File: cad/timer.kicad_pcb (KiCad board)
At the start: 2 copper layers, 47 x 47 mm, 29 parts, among them Q1 BS170, Q2 BS170, U1 ATMEGA328P-PU, U2 LM393, Y1 32.768kHz

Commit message: Further changes from latest KiCad version
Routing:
- net Net-(C8-Pad1): track 8.41 -> 7.56 mm
- net Net-(C9-Pad1): track 8.41 -> 7.57 mm
- net GND: track 34.4 -> 33.9 mm
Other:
- net class Default removed

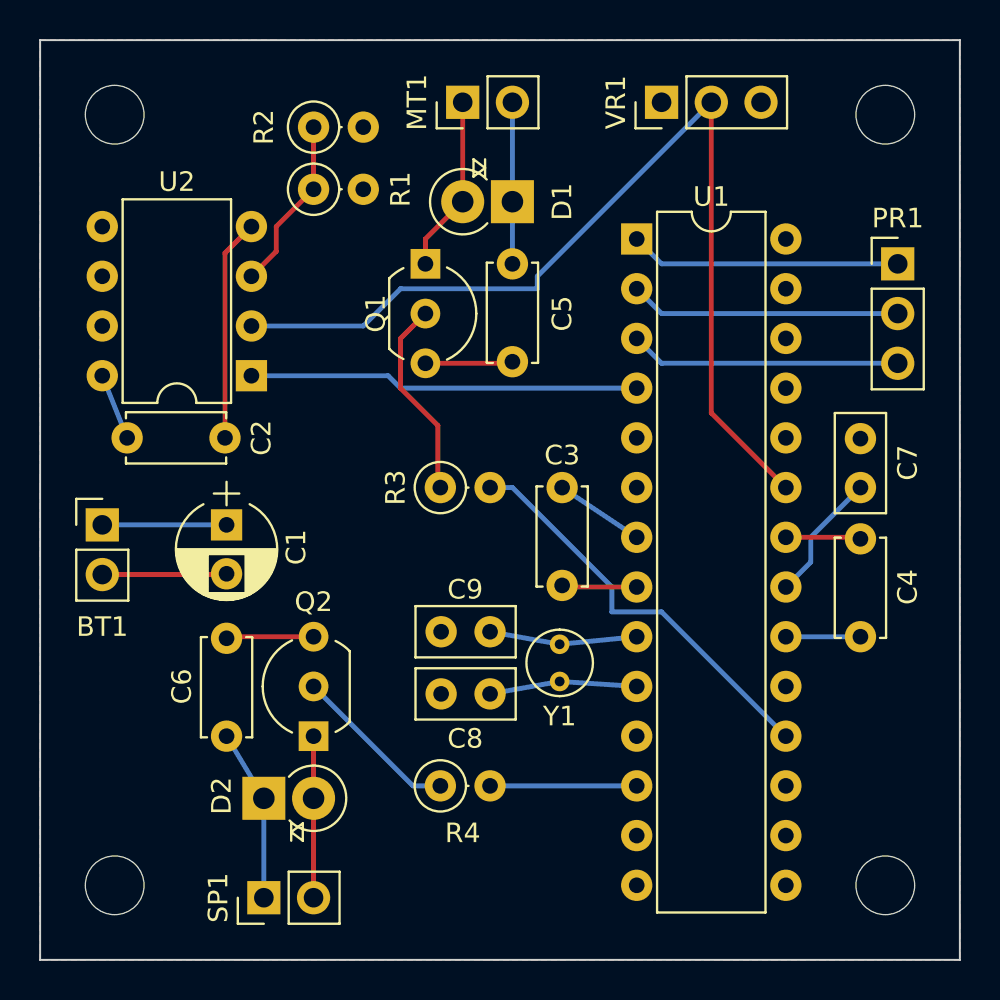
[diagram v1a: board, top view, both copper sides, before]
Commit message: Update CAD for redesign
Also cleanup old files in cad directory
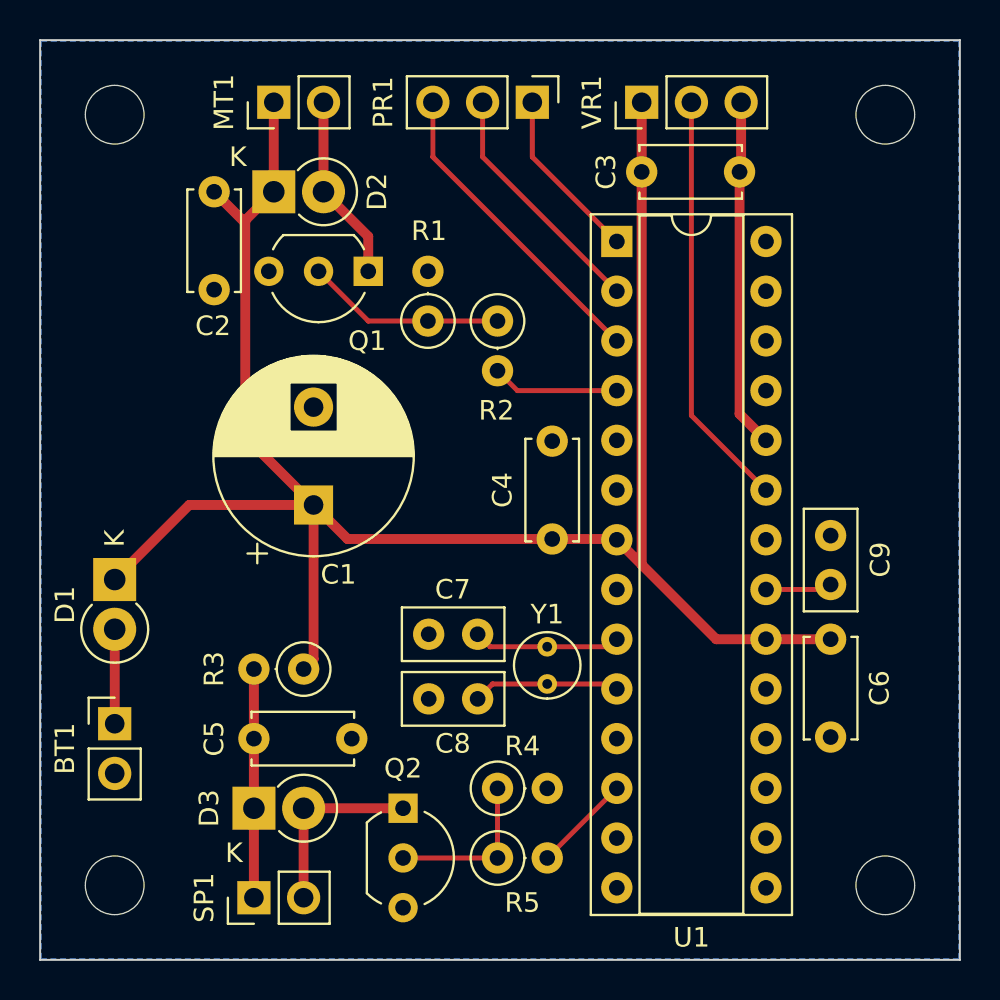
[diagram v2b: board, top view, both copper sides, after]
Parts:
- removed the C2 at (126.4, 89.5)
- removed the R2 at (135.9, 73.7)
- removed U2: LM393, Housings_DIP:DIP-8_W7.62mm
- added C3: 100nF, Capacitor_THT:C_Disc_D5.0mm_W2.5mm_P5.00mm, F.Cu at (152.7, 75.9)
- added D1: 1N5819, Diode_THT:D_DO-41_SOD81_P2.54mm_Vertical_KathodeUp, F.Cu at (125.7, 96.8)
- added R3: 4.7Ω, Resistor_THT:R_Axial_DIN0207_L6.3mm_D2.5mm_P2.54mm_Vertical, F.Cu at (135.4, 101.3)
- added R4: 100kΩ, Resistor_THT:R_Axial_DIN0207_L6.3mm_D2.5mm_P2.54mm_Vertical, F.Cu at (145.3, 107.4)
- BT1, MT1, SP1: footprint Pin_Headers:Pin_Header_Straight_1x02_Pitch2.54mm -> Connector_PinHeader_2.54mm:PinHeader_1x02_P2.54mm_Vertical
- C1: value 10uF -> 470µF; footprint Capacitors_THT:CP_Radial_D5.0mm_P2.50mm -> Capacitor_THT:CP_Radial_D10.0mm_P5.00mm
- C2: renamed from C5; footprint Capacitors_THT:C_Disc_D5.0mm_W2.5mm_P5.00mm -> Capacitor_THT:C_Disc_D5.0mm_W2.5mm_P5.00mm
- C4: renamed from C3; footprint Capacitors_THT:C_Disc_D5.0mm_W2.5mm_P5.00mm -> Capacitor_THT:C_Disc_D5.0mm_W2.5mm_P5.00mm
- C5: renamed from C6; footprint Capacitors_THT:C_Disc_D5.0mm_W2.5mm_P5.00mm -> Capacitor_THT:C_Disc_D5.0mm_W2.5mm_P5.00mm
- C6: renamed from C4; footprint Capacitors_THT:C_Disc_D5.0mm_W2.5mm_P5.00mm -> Capacitor_THT:C_Disc_D5.0mm_W2.5mm_P5.00mm
- C7: renamed from C9; footprint Capacitors_THT:C_Disc_D5.0mm_W2.5mm_P2.50mm -> Capacitor_THT:C_Disc_D5.0mm_W2.5mm_P2.50mm
- C8: footprint Capacitors_THT:C_Disc_D5.0mm_W2.5mm_P2.50mm -> Capacitor_THT:C_Disc_D5.0mm_W2.5mm_P2.50mm
- C9: renamed from C7; footprint Capacitors_THT:C_Disc_D5.0mm_W2.5mm_P2.50mm -> Capacitor_THT:C_Disc_D5.0mm_W2.5mm_P2.50mm
- D2: renamed from D1; footprint Diodes_THT:D_DO-41_SOD81_P2.54mm_Vertical_KathodeUp -> Diode_THT:D_DO-41_SOD81_P2.54mm_Vertical_KathodeUp
- D3: renamed from D2; footprint Diodes_THT:D_DO-41_SOD81_P2.54mm_Vertical_KathodeUp -> Diode_THT:D_DO-41_SOD81_P2.54mm_Vertical_KathodeUp
- PR1, VR1: footprint Pin_Headers:Pin_Header_Straight_1x03_Pitch2.54mm -> Connector_PinHeader_2.54mm:PinHeader_1x03_P2.54mm_Vertical
- Q1, Q2: footprint TO_SOT_Packages_THT:TO-92_Inline_Wide -> Package_TO_SOT_THT:TO-92_Inline_Wide
- R1: value 1MΩ -> 100kΩ; footprint Resistors_THT:R_Axial_DIN0207_L6.3mm_D2.5mm_P2.54mm_Vertical -> Resistor_THT:R_Axial_DIN0207_L6.3mm_D2.5mm_P2.54mm_Vertical
- R2: renamed from R3; value 220Ω -> 1kΩ; footprint Resistors_THT:R_Axial_DIN0207_L6.3mm_D2.5mm_P2.54mm_Vertical -> Resistor_THT:R_Axial_DIN0207_L6.3mm_D2.5mm_P2.54mm_Vertical
- R5: renamed from R4; value 220Ω -> 1kΩ; footprint Resistors_THT:R_Axial_DIN0207_L6.3mm_D2.5mm_P2.54mm_Vertical -> Resistor_THT:R_Axial_DIN0207_L6.3mm_D2.5mm_P2.54mm_Vertical
- U1: footprint Housings_DIP:DIP-28_W7.62mm -> Package_DIP:DIP-28_W7.62mm_Socket
- Y1: footprint Crystals:Crystal_C38-LF_d3.0mm_l8.0mm_Vertical -> Crystal:Crystal_C38-LF_D3.0mm_L8.0mm_Vertical
- moved PR1 20.4 mm to (147.1, 72.4), turned to -90 degrees
- moved C2 15.7 mm to (130.8, 77.0)
- moved D2 12.2 mm to (133.9, 77.0), turned to 0 degrees
- moved BT1 10.2 mm to (125.7, 104.1)
- moved MT1 9.65 mm to (133.9, 72.4)
- moved R2 9.00 mm to (145.3, 83.6), turned to -90 degrees
- moved R1 8.91 mm to (141.7, 83.6), turned to 90 degrees
- moved Q2 5.87 mm to (140.5, 108.5), turned to -90 degrees
- moved C9 5.18 mm to (162.3, 97.0)
- moved R5 4.70 mm to (145.3, 111.0)
- moved C1 4.56 mm to (135.9, 93.0), turned to 90 degrees
- moved Q1 2.95 mm to (138.7, 81.0), turned to 180 degrees
- moved C4 2.68 mm to (148.1, 94.7), turned to 90 degrees
- moved C6 1.53 mm to (162.3, 99.8), turned to -90 degrees
- moved C5 1.40 mm to (132.8, 104.9), turned to 0 degrees
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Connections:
- BT1 pad 1: VCC -> Net-(BT1-Pad1)
- C5 pad 1: VCC -> Net-(C5-Pad1)
- D2 pad 2: Net-(D1-Pad2) -> Net-(D2-Pad2)
- D3 pad 1: VCC -> Net-(C5-Pad1)
- MT1 pad 1: Net-(D1-Pad2) -> VCC
- MT1 pad 2: VCC -> Net-(D2-Pad2)
- Q1 pad 1: Net-(D1-Pad2) -> Net-(D2-Pad2)
- R1 pad 1: Net-(R1-Pad1) -> Net-(Q1-Pad2)
- R1 pad 2: VCC -> GND
- R2 pad 2: Net-(R3-Pad2) -> Net-(U1-Pad4)
- SP1 pad 1: VCC -> Net-(C5-Pad1)
- U1 pad 11: Net-(U1-Pad11) -> unconnected-(U1-Pad11)
- U1 pad 13: Net-(U1-Pad13) -> unconnected-(U1-Pad13)
- U1 pad 14: Net-(U1-Pad14) -> unconnected-(U1-Pad14)
- U1 pad 15: Net-(U1-Pad15) -> unconnected-(U1-Pad15)
- U1 pad 16: Net-(U1-Pad16) -> unconnected-(U1-Pad16)
- U1 pad 17: Net-(U1-Pad17) -> unconnected-(U1-Pad17)
- U1 pad 18: Net-(R3-Pad2) -> unconnected-(U1-Pad18)
- U1 pad 19: Net-(U1-Pad19) -> unconnected-(U1-Pad19)
- U1 pad 24: Net-(U1-Pad24) -> Net-(C3-Pad2)
- U1 pad 25: Net-(U1-Pad25) -> unconnected-(U1-Pad25)
- U1 pad 26: Net-(U1-Pad26) -> unconnected-(U1-Pad26)
- U1 pad 27: Net-(U1-Pad27) -> unconnected-(U1-Pad27)
- U1 pad 28: Net-(U1-Pad28) -> unconnected-(U1-Pad28)
- U1 pad 5: Net-(U1-Pad5) -> unconnected-(U1-Pad5)
- U1 pad 6: Net-(U1-Pad6) -> unconnected-(U1-Pad6)
- VR1 pad 3: GND -> Net-(C3-Pad2)
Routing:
- net VCC: track 35.2 -> 98.0 mm
- net GND: track 33.9 -> 0.00 mm
- net Net-(U1-Pad23): track 49.9 -> 21.4 mm
- net Net-(R3-Pad2): track 21.1 -> 0.00 mm
- net Net-(C3-Pad2): track 0.00 -> 17.8 mm
- net Net-(U1-Pad4): track 19.9 -> 6.52 mm
- net Net-(C5-Pad1): track 0.00 -> 11.7 mm
- net Net-(D2-Pad2): track 0.00 -> 9.58 mm
- net Net-(D1-Pad2): track 9.04 -> 0.00 mm
- net Net-(R1-Pad1): track 8.94 -> 0.00 mm
- net Net-(PR1-Pad1): track 13.9 -> 8.90 mm
- net Net-(BT1-Pad1): track 0.00 -> 4.83 mm
- net Net-(C9-Pad1): track 6.66 -> 3.05 mm
- net Net-(R5-Pad2): track 7.49 -> 5.03 mm
- net Net-(PR1-Pad3): track 13.9 -> 16.1 mm
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- added copper zone on B.Cu, net GND
- removed copper zone on F.Cu, net GND
- removed copper zone on B.Cu, net VCC
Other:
- rule pad_to_mask_clearance: 0.2 -> 0
